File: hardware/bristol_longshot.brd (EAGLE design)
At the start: 12 x 55 mm, 42 parts, among them U1 SAM_D20E, U2 SI4060, U3 MAX1947, U4 ANTENOVA_GPS_M10382, U5 S25FS-S

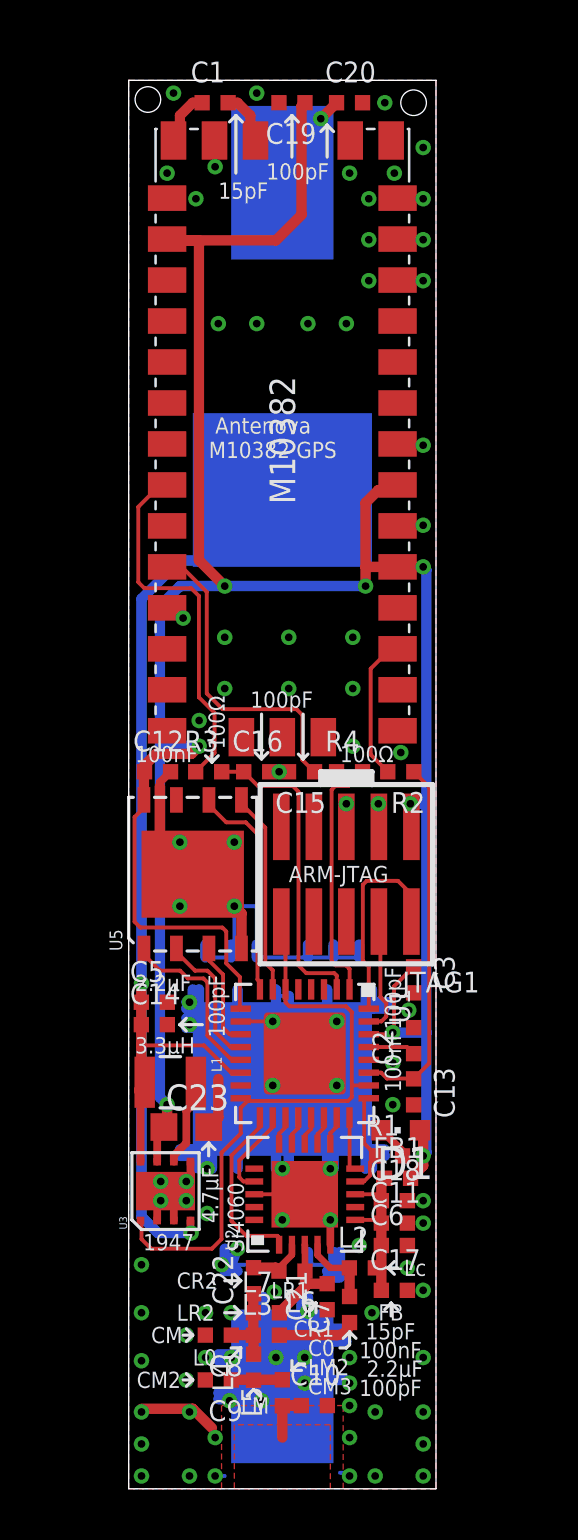
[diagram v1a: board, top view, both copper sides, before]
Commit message: Board revision 0.96.0 sent
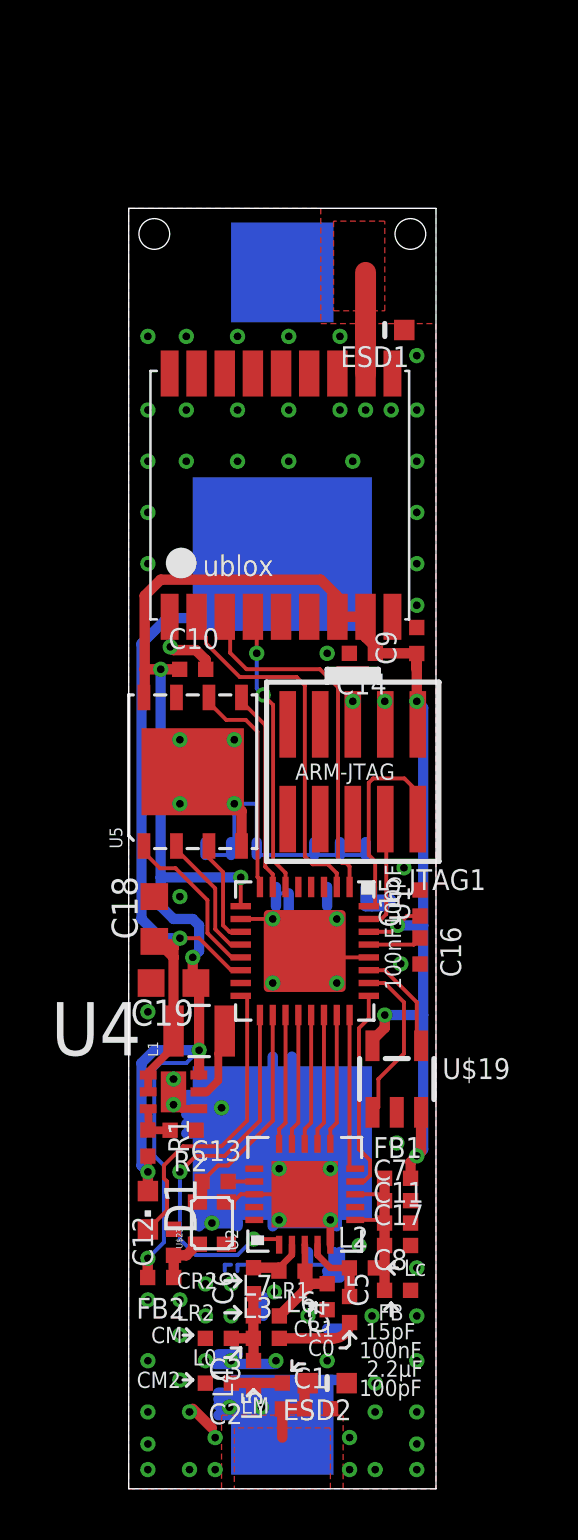
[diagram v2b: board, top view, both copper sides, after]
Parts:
- removed C20: 100pF, microbuilder_v3:_0402
- removed C21: 15pF, microbuilder_v3:_0402
- removed C22: DNP, microbuilder_v3:_0402
- removed C23: 4.7µF, resistor:C0603K
- removed R3, R4: 100Ω, microbuilder_v3:_0402
- removed U3: MAX1947, fbri:TDFN8
- added C4: 15pF, microbuilder_v3:_0402
- added ESD1, ESD2: 0.25pF, microbuilder_v3:_0603MP
- added FB2: (no value), microbuilder_v3:_0402
- added U$19: TPS3123, TPS3125:SOT23-5
- added U$23: TG-5006CJ, fbri:TC-5006CJ
- added U$48: UBLOX_MAX, Ava:UBLOX_MAX
- C1: value 15pF -> 8.2pF
- C10, C8: value 8.2pF -> 100pF
- C13, C14, C15, C16: value 100pF -> 100nF
- C17: value 100pF -> 2.2µF
- C18: value 15pF -> 10µF; device microbuilder_v3:_0402 -> resistor:C0603K
- C19: value 100pF -> 10µF; device microbuilder_v3:_0402 -> resistor:C0603K
- C2: value 100nF -> 15pF
- C3: value 100nF -> 8.2pF
- C5, C6: value 2.2µF -> DNP
- C9: value 15pF -> 100pF
- L1: value 3.3µH -> 2.2µH
- R1: value 22Ω -> 100kΩ
- R2: value 100Ω -> 240kΩ
- U4: value ANTENOVA_GPS_M10382 -> ADP1607ACPZN-R7; device fbri:ANTENOVA_GPS_M10382 -> ADP1607:DFN200X200X60-7N
- moved C1 51.2 mm to (7.38, 3.12)
- moved C19 34.7 mm to (1.75, 19.8)
- moved C9 29.9 mm to (11.2, 33.1), turned to 90 degrees
- moved C10 29.1 mm to (2.50, 32.0)
- moved U4 25.9 mm to (1.75, 15.5)
- moved C12 18.4 mm to (1.75, 9.62), turned to 90 degrees
- moved C14 16.6 mm to (9.12, 32.6), turned to 180 degrees
- moved R2 16.4 mm to (2.12, 14.0)
- moved C3 15.9 mm to (3.50, 5.88), turned to 180 degrees
- moved C2 15.4 mm to (3.50, 4.12), turned to 180 degrees
- moved C18 14.5 mm to (1.00, 22.2), turned to 90 degrees
- moved C5 13.3 mm to (7.75, 7.50), turned to 270 degrees
- moved D1 10.4 mm to (0.75, 10.9), turned to 180 degrees
- moved C16 9.47 mm to (11.4, 21.0), turned to 270 degrees
- moved R1 9.45 mm to (0.75, 13.5), turned to 270 degrees
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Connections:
- removed net AN_GPS_RX: C15.1, R4.1, U4.13_RX
- removed net AN_GPS_TX: R3.1, U4.11_TX
- removed net GPS_ANT_IN: C1.2, U4.1_ANT_IN
- removed net GPS_ANT_OUT: C1.1, U4.3_ANT_OUT
- removed net GPS_RX: R4.2, U1.1
- removed net GPS_TX: C16.1, R3.2, U1.2
- removed net LED_RES: D1.C, R1.2
- removed net LX: L1.1, U3.6
- removed net N$1: C20.1, U$2.+1
- removed net RESETN: JTAG1.10, U1.16, U1.26, U1.6, U3.1
- removed net SI_HF_CLK: U1.18, U2.17
- removed net TIME_1KHZ: C13.1, R2.1, U1.27
- removed net TIME_1KHZ_DRIVE: R2.2, U4.23_TIMEPULSE/TDO
- new net !RESET: U$19.1, U1.26
- new net +2: U$2.+1
- new net 9_V_RESET: U$48.9_V_RESET
- new net FB: R1.1, R2.2, U4.3
- new net GIMO: U$48.3_RXD1, U1.1
- new net GOMI: U$48.2_TXD1, U1.2
- new net GPS_ANT: ESD1.2, U$48.11_RF_IN
- new net LED: D1.C, U1.16
- new net RADIO_XIN: C13.2, U2.17
- new net SW: L1.2, U4.5
- new net TCXO_OUT: C13.1, U$23.3, U1.18
- new net TCXO_VDD: C12.1, FB2.1, U$23.4
- new net TIMEPULSE: U$48.4_TIMEPULSE, U1.6
- new net WDI: U$19.4, U1.27
- net 1.2V: now also C18.1, L1.1, U4.1, U4.2; no longer C14.1, C5.1, L1.2, U3.4, U3.8
- net 1.8V: now also C10.1, C14.1, C15.1, C9.1, FB2.2, R1.2, U$19.3, U$19.5, U$48.7_VCC_IO, U$48.8_VCC, U4.6; no longer C12.1, C23.1, C3.1, U3.7, U4.25_VDD_RF, U4.27_VCC, U4.5_VIO
- net ANT: now also C1.1, ESD2.2; no longer C10.1
- net FILTER1: now also C3.1, C6.1; no longer C22.1, C8.1
- net FILTER2: now also C2.1; no longer C9.1
- net GND: now also C1.2, C7.2, ESD1.1, ESD2.1, R2.1, U$19.2, U$23.2, U$48.10_GND, U$48.12_GND, U$48.1_GND, U4.4, U4.7; no longer C13.2, C20.2, C21.1, C23.2, C6.2, U3.2, U3.3, U3.5, U3.PAD, U4.14_GND, U4.17_GND, U4.21_GND, U4.24_GND, U4.26_GND, U4.28_GND, U4.2_GND, U4.32_VDD_USB, U4.33_GND, U4.34_GND, U4.35_GND, U4.36_GND, U4.4_GND
- net RADIO_VDD: now also C7.1, C8.1; no longer C18.1, C6.1
- net RF_OUT: now also C4.2; no longer C7.2
- net RXN: now also C5.1; no longer C21.2
- net RXP: now also C6.2; no longer C22.2
- net SI_GPIO0: no longer R1.1
- net TANK: now also C4.1; no longer C7.1
- net VDD_CORE: now also C16.1; no longer C2.1
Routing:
- net RESETN: track 24.5 -> 0.00 mm
- net 1.8V: track 113.0 -> 89.3 mm, vias 8 -> 10
- net 1.2V: track 45.8 -> 30.5 mm, vias 2 -> 1
- net AN_GPS_TX: track 14.6 -> 0.00 mm
- net GOMI: track 0.00 -> 14.5 mm
- net TIME_1KHZ: track 14.3 -> 0.00 mm
- net GIMO: track 0.00 -> 14.3 mm
- net AN_GPS_RX: track 13.3 -> 0.00 mm
- net GPS_TX: track 12.3 -> 0.00 mm
- net LED: track 0.00 -> 12.0 mm
- net TIMEPULSE: track 0.00 -> 11.0 mm, vias 0 -> 2
- net GPS_RX: track 9.83 -> 0.00 mm
- net TCXO_OUT: track 0.00 -> 8.74 mm
- net SI_SDN: track 7.10 -> 15.5 mm, vias 0 -> 2
- net GND: track 83.9 -> 76.1 mm, vias 99 -> 87
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- added copper zone on layer 1, net GPS_ANT
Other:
- board size 12 x 55 mm -> 12 x 50 mm
- board text added: "BRISTOL"
- board text added: "GPS"
- board text added: "OF"
- board text added: "UNIVERSITY"
- board text added: "ublox"
- board text added: "v0.96.0"
- board text removed: "100nF"
- board text removed: "100pF"
- board text removed: "100Ω"
- board text removed: "15pF"
- board text removed: "1947"
- board text removed: "3.3µH"
- board text removed: "4.7µF"
- board text removed: "Antenova M10382 GPS"
- board text removed: "Bristol"
- board text removed: "CM3"
- board text removed: "LM2"
- board text removed: "Longshot"
- board text removed: "Si4060"
- board text removed: "Version 0.95.0"
